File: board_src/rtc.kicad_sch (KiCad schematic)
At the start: 10 parts, among them IC1 PCF8563TS_4,118, J9 Conn_01x02_Pin, Y2 Crystal

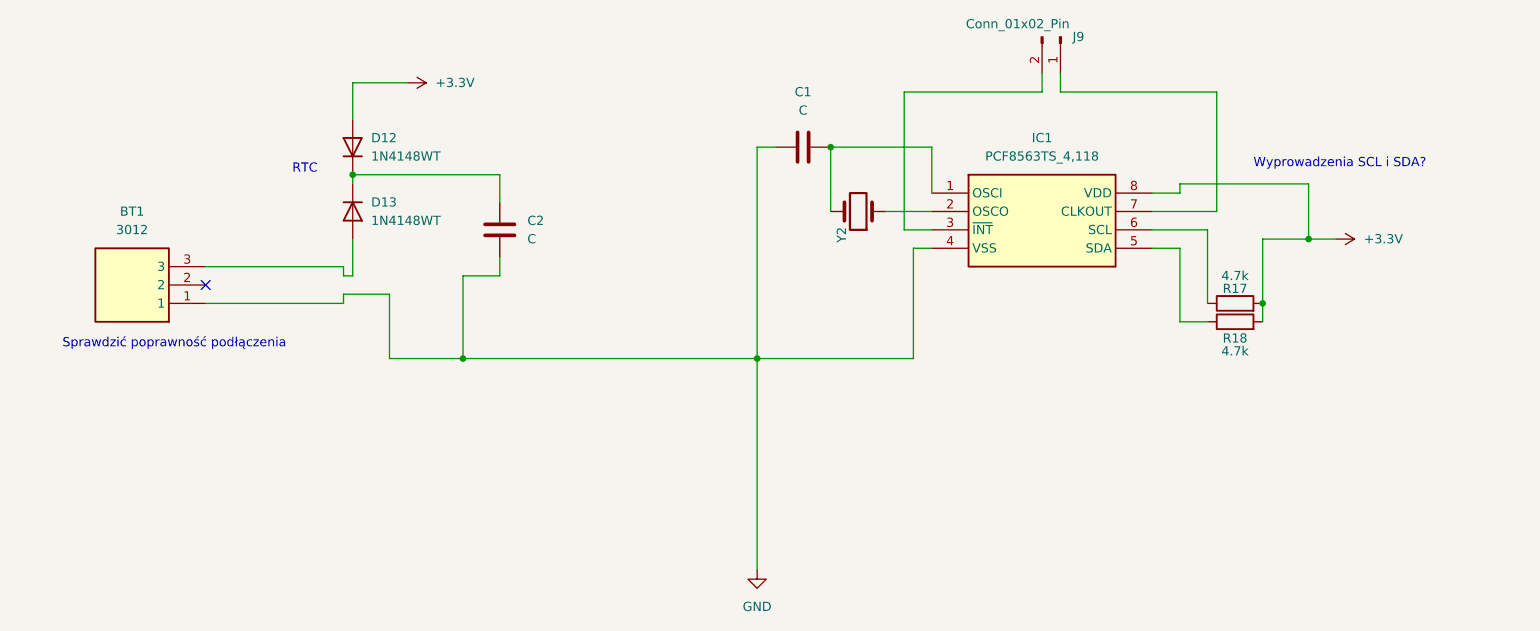
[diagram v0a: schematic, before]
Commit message: wersja z FT232RN
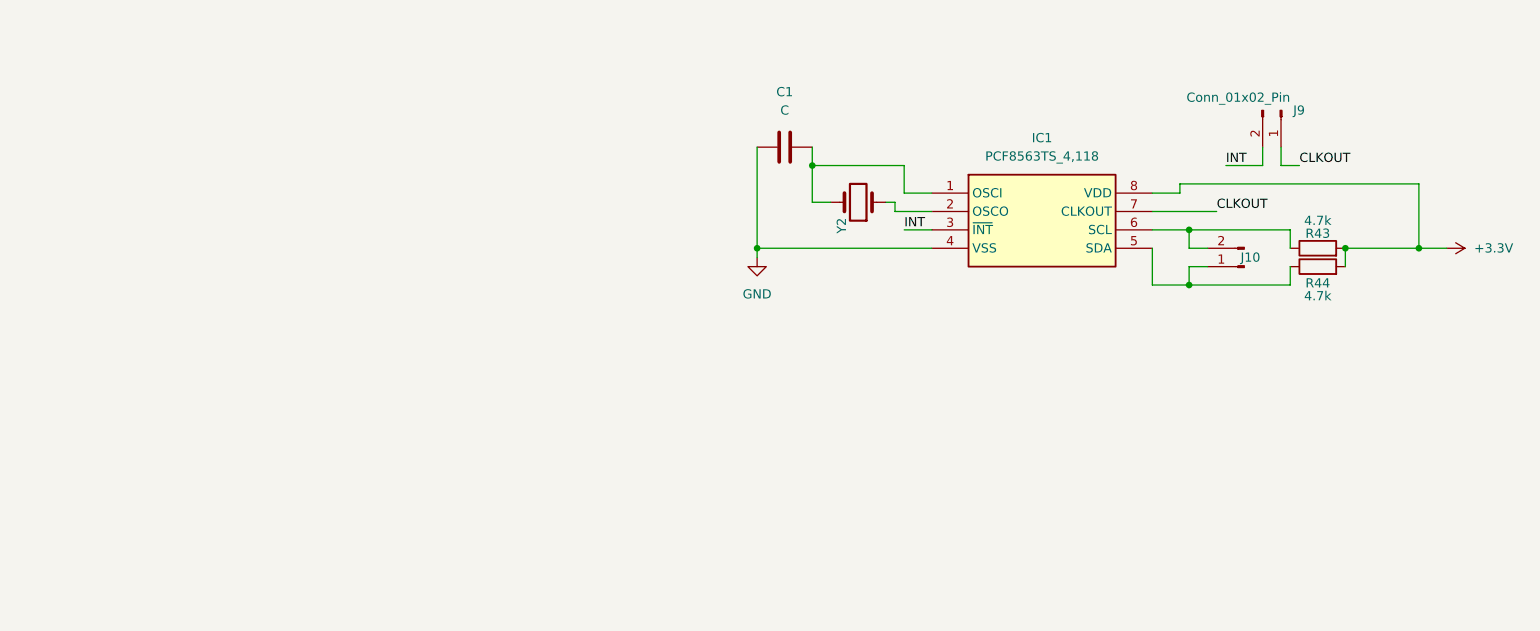
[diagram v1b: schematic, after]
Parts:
- removed BT1: 3012, footprints:3012, symbol 3012:3012
- removed C2: C, Capacitor_SMD:C_0201_0603Metric, symbol Device:C
- removed D12, D13: 1N4148WT, Diode_SMD:D_SOD-523, symbol Diode:1N4148WT
- removed R17, R18: 4.7k, Resistor_SMD:R_0201_0603Metric, symbol Device:R
- added J10: Conn_01x02_Pin, Connector_PinHeader_2.54mm:PinHeader_1x02_P2.54mm_Vertical, symbol Connector:Conn_01x02_Pin
- added R43, R44: 4.7k, Resistor_SMD:R_1206_3216Metric, symbol Device:R
- C1: footprint Capacitor_SMD:C_0201_0603Metric -> Capacitor_SMD:C_1206_3216Metric
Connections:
- net +3.3V: now also R43.2, R44.2
- net at IC1.5 (SDA): now also J10.1 (Pin_1), R44.1
- net INT: now reaches IC1.3 (~{INT}), J9.2 (Pin_2)
- net at IC1.6 (SCL): now also J10.2 (Pin_2), R43.1
- net CLKOUT: now reaches IC1.7 (CLKOUT), J9.1 (Pin_1)
- no-connect marks 1 -> 0
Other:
- note removed: "RTC"
- note removed: "Sprawdzić poprawność podłączenia"
- note removed: "Wyprowadzenia SCL i SDA?"
- moved on the sheet: C1, J9, Y2
